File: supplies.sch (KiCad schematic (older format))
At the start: 17 parts, among them U1 L7805, U2 AMS1117-3.3

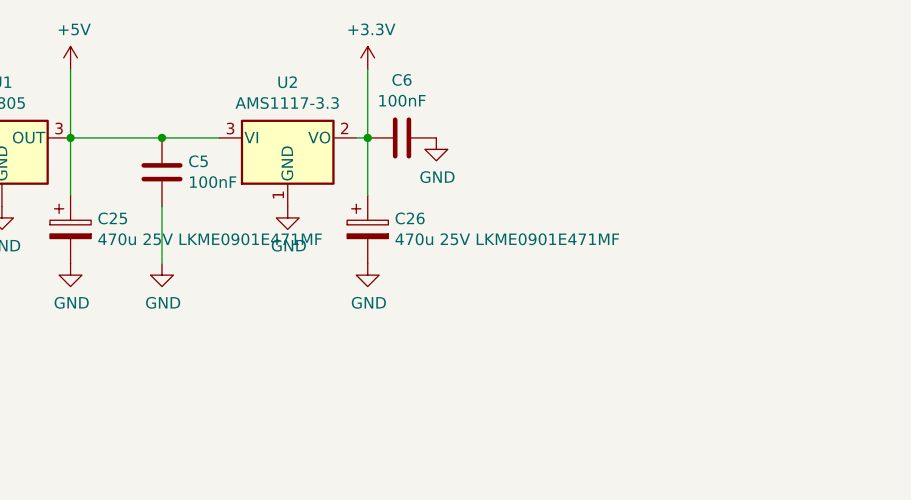
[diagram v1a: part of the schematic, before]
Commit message: Add +3.3V reverse current protection diode; add +3.3V on debug header
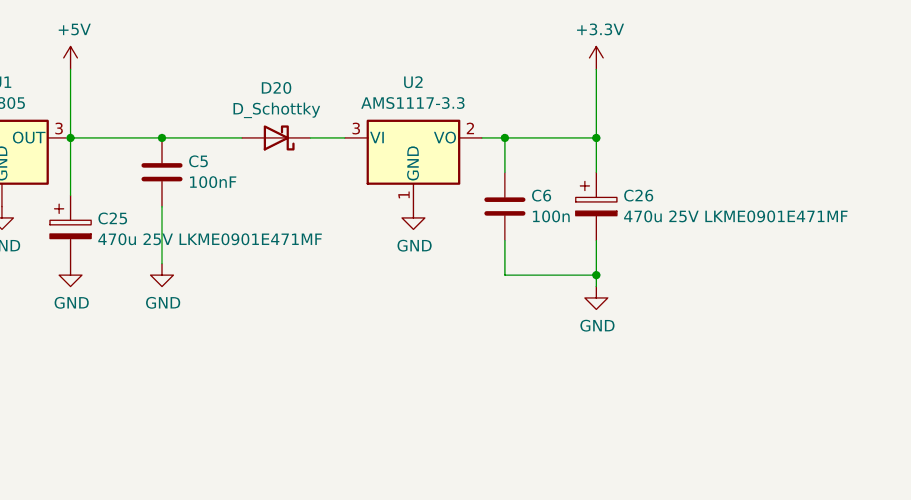
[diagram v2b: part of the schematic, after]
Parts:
- added D20: D_Schottky, symbol Device:D_Schottky
- C6: value 100nF -> 100n; footprint Capacitor_SMD:C_0603_1608Metric -> (none)
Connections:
- net +3V3: now also C6.1; no longer C6.2
- net +5V: now also D20.2 (A); no longer U2.3 (VI)
- net GND: now also C6.2; no longer C6.1
- new net: D20.1 (K), U2.3 (VI)
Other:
- moved on the sheet: C26, U2
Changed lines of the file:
@@
 L Regulator_Linear:AMS1117-3.3 U2
 U 1 1 5F73F583
-P 8600 1450
-F 0 "U2" H 8600 1692 50  0000 C CNN
-F 1 "AMS1117-3.3" H 8600 1601 50  0000 C CNN
-F 2 "Package_TO_SOT_SMD:SOT-223-3_TabPin2" H 8600 1650 50  0001 C CNN
-F 3 "http://www.advanced-monolithic.com/pdf/ds1117.pdf" H 8700 1200 50  0001 C CNN
-	1    8600 1450
+P 9150 1450
+F 0 "U2" H 9150 1692 50  0000 C CNN
+F 1 "AMS1117-3.3" H 9150 1601 50  0000 C CNN
+F 2 "Package_TO_SOT_SMD:SOT-223-3_TabPin2" H 9150 1650 50  0001 C CNN
+F 3 "http://www.advanced-monolithic.com/pdf/ds1117.pdf" H 9250 1200 50  0001 C CNN
+	1    9150 1450
 	1    0    0    -1
 $EndComp
@@
 L Device:CP C26
 U 1 1 5F7432C1
-P 8950 1850
-F 0 "C26" H 9068 1896 50  0000 L CNN
-F 1 "470u 25V LKME0901E471MF" H 9068 1805 50  0000 L CNN
-F 2 "Capacitor_THT:CP_Radial_D10.0mm_P5.00mm" H 8988 1700 50  0001 C CNN
-F 3 "~" H 8950 1850 50  0001 C CNN
-	1    8950 1850
+P 9950 1750
+F 0 "C26" H 10068 1796 50  0000 L CNN
+F 1 "470u 25V LKME0901E471MF" H 10068 1705 50  0000 L CNN
+F 2 "Capacitor_THT:CP_Radial_D10.0mm_P5.00mm" H 9988 1600 50  0001 C CNN
+F 3 "~" H 9950 1750 50  0001 C CNN
+	1    9950 1750
 	1    0    0    -1
 $EndComp
@@
 	7650 1450 7650 1700
 Wire Wire Line
-	8900 1450 8950 1450
-Wire Wire Line
-	8950 1450 8950 1700
+	9950 1450 9950 1600
 $Comp
 L power:GND #PWR0123
 U 1 1 5F7440BE
-P 8950 2000
-F 0 "#PWR0123" H 8950 1750 50  0001 C CNN
-F 1 "GND" H 8955 1827 50  0000 C CNN
-F 2 "" H 8950 2000 50  0001 C CNN
-F 3 "" H 8950 2000 50  0001 C CNN
-	1    8950 2000
+P 9950 2100
+F 0 "#PWR0123" H 9950 1850 50  0001 C CNN
+F 1 "GND" H 9955 1927 50  0000 C CNN
+F 2 "" H 9950 2100 50  0001 C CNN
+F 3 "" H 9950 2100 50  0001 C CNN
+	1    9950 2100
 	1    0    0    -1
 $EndComp
@@
 L power:GND #PWR0124
 U 1 1 5F7441D8
-P 8600 1750
-F 0 "#PWR0124" H 8600 1500 50  0001 C CNN
-F 1 "GND" H 8605 1577 50  0000 C CNN
-F 2 "" H 8600 1750 50  0001 C CNN
-F 3 "" H 8600 1750 50  0001 C CNN
-	1    8600 1750
+P 9150 1750
+F 0 "#PWR0124" H 9150 1500 50  0001 C CNN
+F 1 "GND" H 9155 1577 50  0000 C CNN
+F 2 "" H 9150 1750 50  0001 C CNN
+F 3 "" H 9150 1750 50  0001 C CNN
+	1    9150 1750
 	1    0    0    -1
 $EndComp
@@
 L power:+3.3V #PWR0127
 U 1 1 5F744EDF
-P 8950 1150
-F 0 "#PWR0127" H 8950 1000 50  0001 C CNN
-F 1 "+3.3V" H 8965 1323 50  0000 C CNN
-F 2 "" H 8950 1150 50  0001 C CNN
-F 3 "" H 8950 1150 50  0001 C CNN
-	1    8950 1150
-	1    0    0    -1
-$EndComp
-Wire Wire Line
-	8950 1150 8950 1450
-Connection ~ 8950 1450
+P 9950 1150
+F 0 "#PWR0127" H 9950 1000 50  0001 C CNN
+F 1 "+3.3V" H 9965 1323 50  0000 C CNN
+F 2 "" H 9950 1150 50  0001 C CNN
+F 3 "" H 9950 1150 50  0001 C CNN
+	1    9950 1150
+	1    0    0    -1
+$EndComp
+Wire Wire Line
+	9950 1150 9950 1450
+Connection ~ 9950 1450
 Text HLabel 3650 1550 0    50   Input ~ 0
 V_BATT_MEAS
@@
 Wire Wire Line
 	7650 1450 8050 1450
-Wire Wire Line
-	8300 1450 8050 1450
 Connection ~ 8050 1450
-$Comp
-L Device:C C6
-U 1 1 5F7529AF
-P 9100 1450
-F 0 "C6" V 8848 1450 50  0000 C CNN
-F 1 "100nF" V 8939 1450 50  0000 C CNN
-F 2 "Capacitor_SMD:C_0603_1608Metric" H 9138 1300 50  0001 C CNN
-F 3 "~" H 9100 1450 50  0001 C CNN
-	1    9100 1450
-	0    1    1    0
-$EndComp
-$Comp
-L power:GND #PWR0130
-U 1 1 5F752FD7
-P 9250 1450
-F 0 "#PWR0130" H 9250 1200 50  0001 C CNN
-F 1 "GND" H 9255 1277 50  0000 C CNN
-F 2 "" H 9250 1450 50  0001 C CNN
-F 3 "" H 9250 1450 50  0001 C CNN
-	1    9250 1450
-	1    0    0    -1
-$EndComp
 $Comp
 L Connector_Generic:Conn_01x05 Buck1
@@
 	1    0    0    -1
 $EndComp
+$Comp
+L Device:D_Schottky D20
+U 1 1 5F877F67
+P 8550 1450
+F 0 "D20" H 8550 1233 50  0000 C CNN
+F 1 "D_Schottky" H 8550 1324 50  0000 C CNN
+F 2 "" H 8550 1450 50  0001 C CNN
+F 3 "~" H 8550 1450 50  0001 C CNN
+	1    8550 1450
+	-1   0    0    1
+$EndComp
+Wire Wire Line
+	8050 1450 8400 1450
+Wire Wire Line
+	8700 1450 8850 1450
+$Comp
+L Device:C C6
+U 1 1 5F87BC4D
+P 9550 1750
+F 0 "C6" H 9665 1796 50  0000 L CNN
+F 1 "100n" H 9665 1705 50  0000 L CNN
+F 2 "" H 9588 1600 50  0001 C CNN
+F 3 "~" H 9550 1750 50  0001 C CNN
+	1    9550 1750
+	1    0    0    -1
+$EndComp
+Wire Wire Line
+	9450 1450 9550 1450
+Wire Wire Line
+	9550 1450 9550 1600
+Wire Wire Line
+	9550 1450 9950 1450
+Connection ~ 9550 1450
+Wire Wire Line
+	9550 1900 9550 2050
+Wire Wire Line
+	9550 2050 9950 2050
+Wire Wire Line
+	9950 2050 9950 1900
+Wire Wire Line
+	9950 2050 9950 2100
+Connection ~ 9950 2050
 $EndSCHEMATC

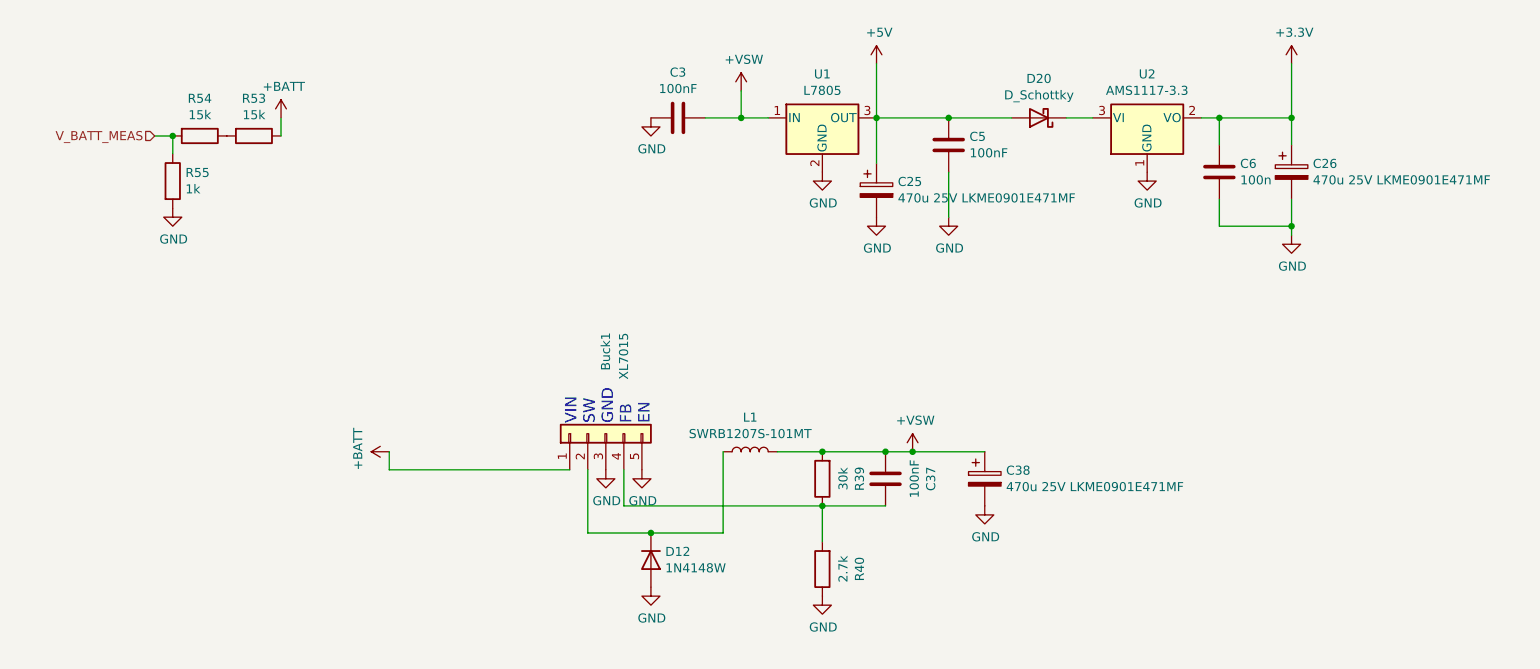
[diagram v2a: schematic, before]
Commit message: Add TVS diode, fuse to 15 V supply
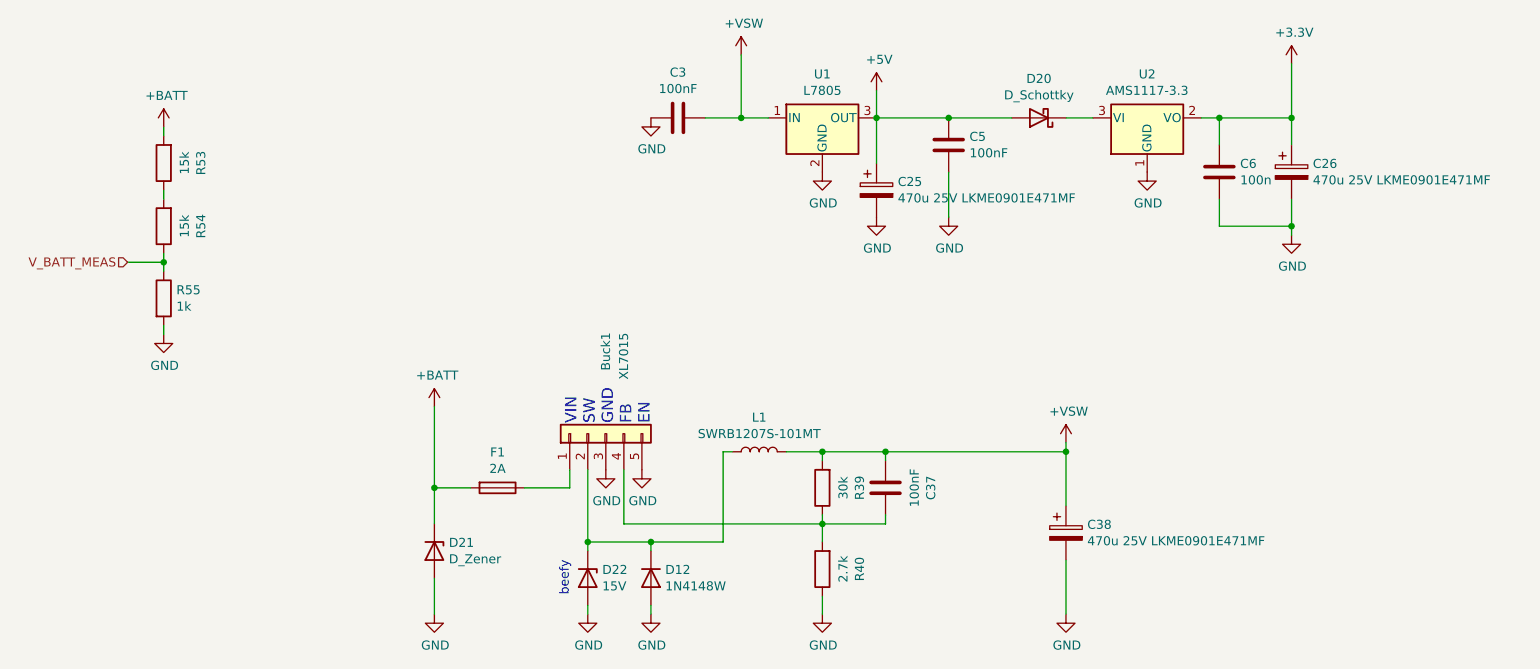
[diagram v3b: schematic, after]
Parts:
- added D21: D_Zener, symbol Device:D_Zener
- added D22: 15V, symbol Device:D_Zener
- added F1: 2A, symbol Device:Fuse
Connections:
- net +BATT: now also R53.2, D21.1 (K), F1.2; no longer Buck1.1 (Pin_1), R53.1
- net GND: now also D21.2 (A), D22.2 (A)
- net V_BATT_MEAS: now also R54.1; no longer R54.2
- net at Buck1.2 (Pin_2), D12.1 (K), L1.1: now also D22.1 (K)
- new net: Buck1.1 (Pin_1), F1.1
- new net: R53.1, R54.2
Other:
- note added: "beefy"
- moved on the sheet: C37, C38, D12, L1, R39, R53, R54, R55
